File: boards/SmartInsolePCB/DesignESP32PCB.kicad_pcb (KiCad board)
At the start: 2 copper layers, 51 x 81.5 mm, 60 parts, among them J1 PJS008U-3000-0, J10 Conn_01x02_Pin, J11 Conn_01x02_Pin, J12 Conn_01x02_Pin, J13 Conn_01x05_Socket, J2 Conn_01x02_Pin, J3 Conn_01x02_Pin, J4 Conn_01x02_Pin, J5 Conn_01x02_Pin, J6 Conn_01x02_Pin, J7 Conn_01x02_Pin, J8 Conn_01x02_Pin, J9 Conn_01x02_Pin, Q1 SS8050-G, Q2 SS8050-G, SW1 B3F-4000, SW2 B3F-4000, SW3 B3F-4000, SW4 B3F-4000, U1 D3V3XA4B10LP, U2 ESP32-S3-WROOM-1, U3 MPU-6050, U4 TLV75801PDRV

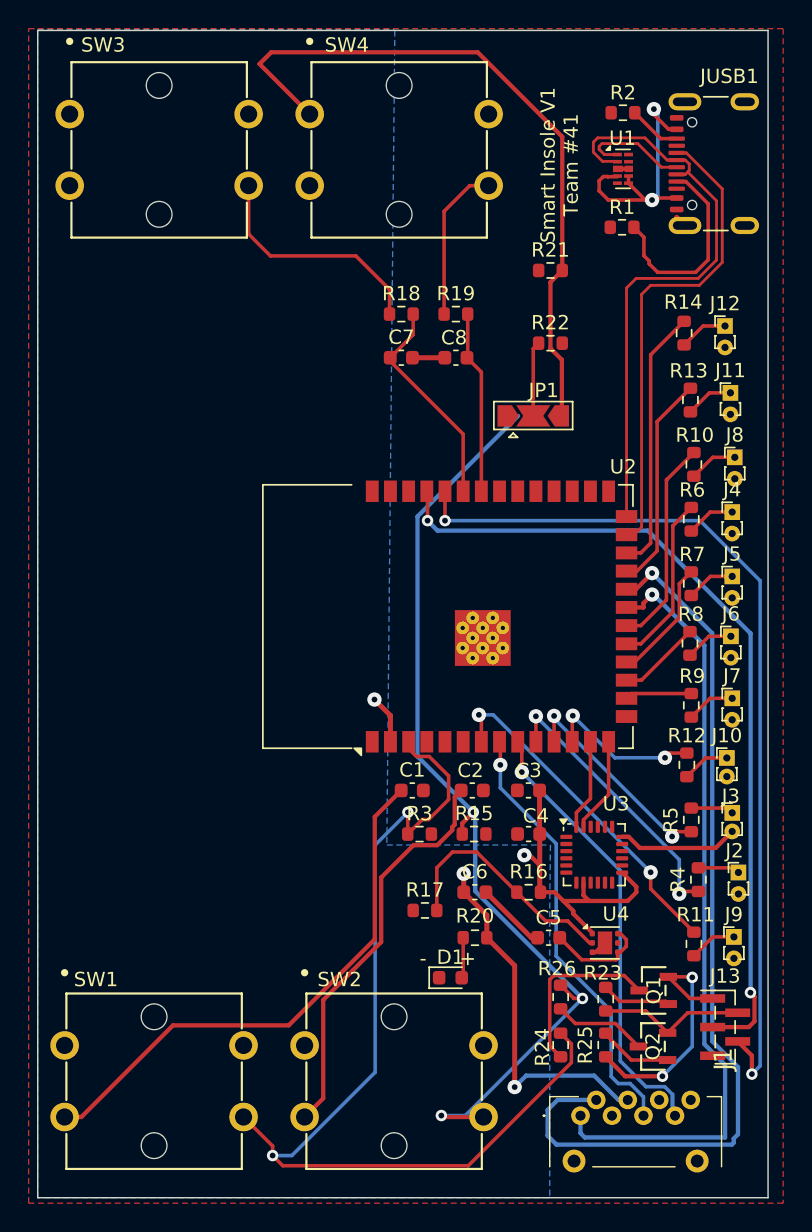
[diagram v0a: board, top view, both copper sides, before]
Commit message: down to 56
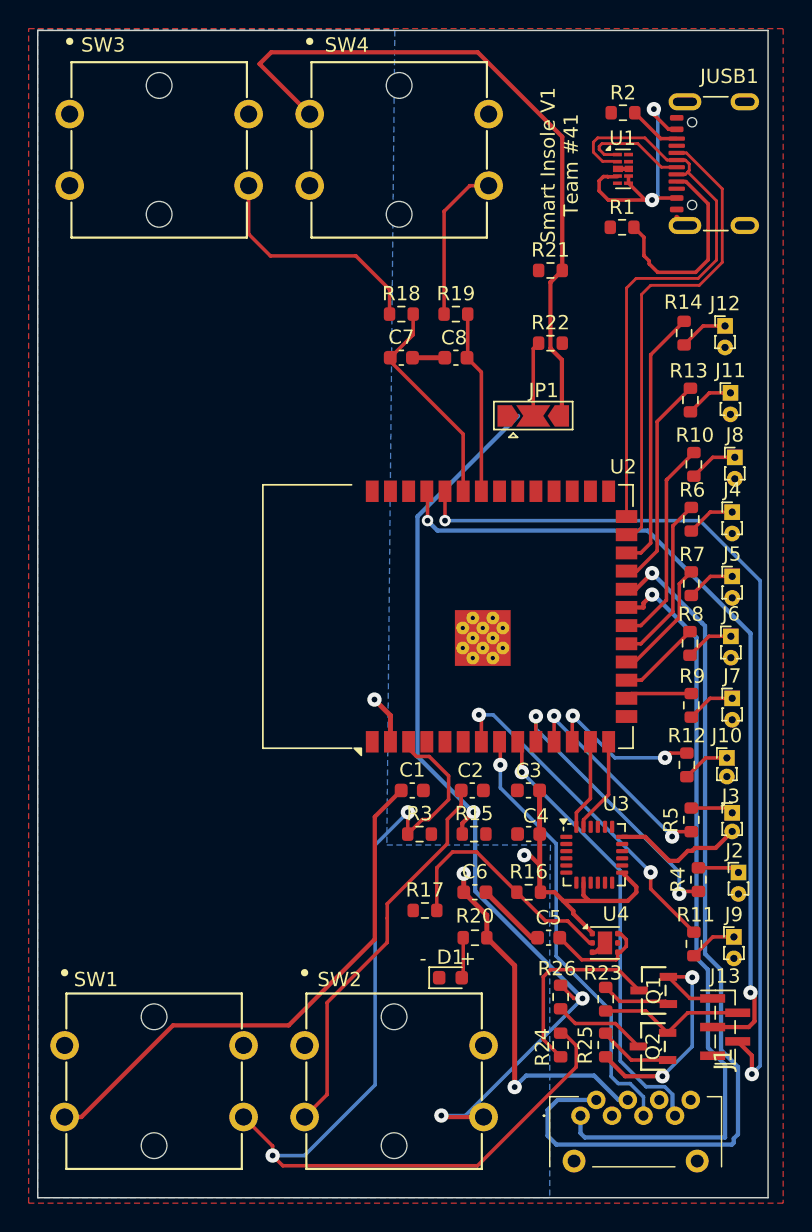
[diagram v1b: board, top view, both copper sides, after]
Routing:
- net /ESP32_EN: track 69.9 -> 71.2 mm
- net Net-(Q1-Pad3): track 12.5 -> 13.6 mm
- net Net-(C2-Pad1): track 28.3 -> 27.3 mm
- net GND: track 18.6 -> 19.3 mm
